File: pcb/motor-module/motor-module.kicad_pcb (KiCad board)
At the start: 2 copper layers, 37 x 27 mm, 9 parts, among them J1 Connector_male, J2 Screw_Terminal_01x02, K1 AZ822-2C-5DSE Signal-Relais, 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, Q1 2N 2222A SMD Bipolartransisto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

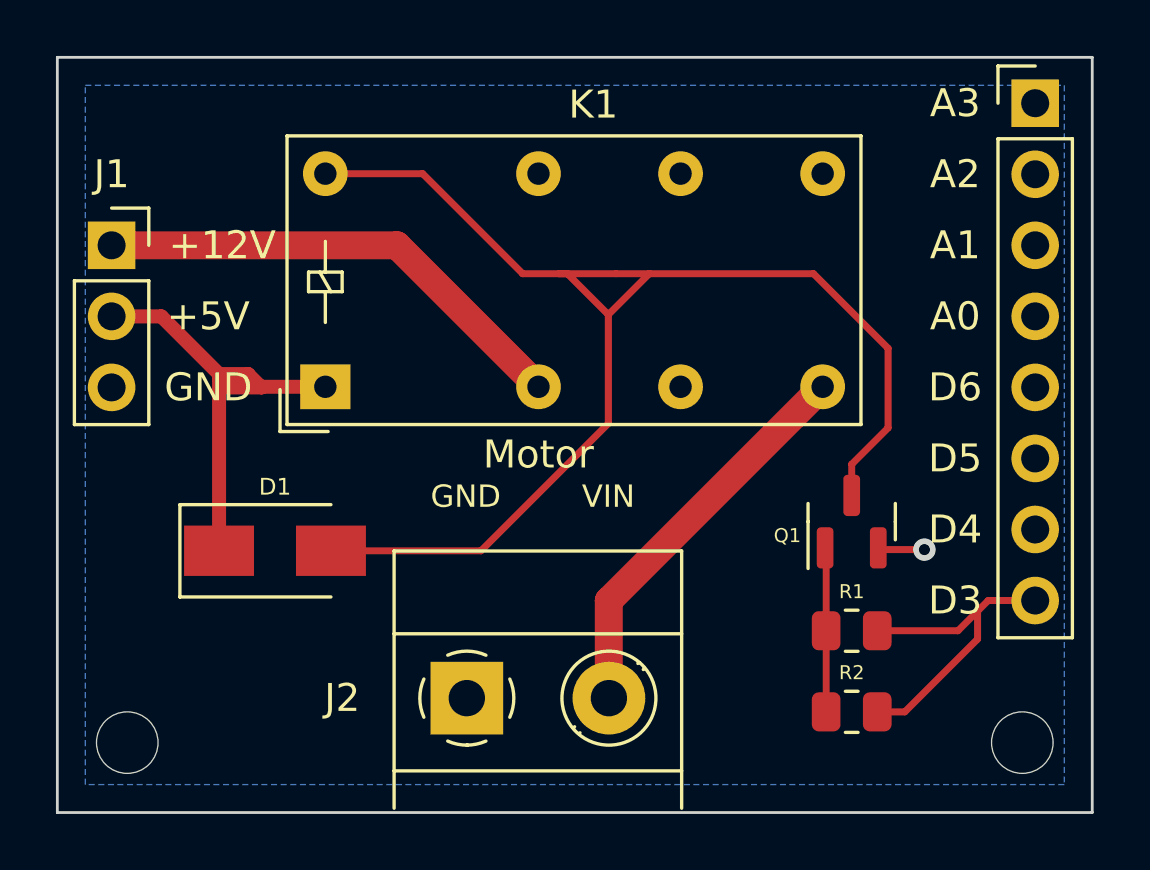
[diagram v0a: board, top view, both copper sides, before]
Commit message: pcb update
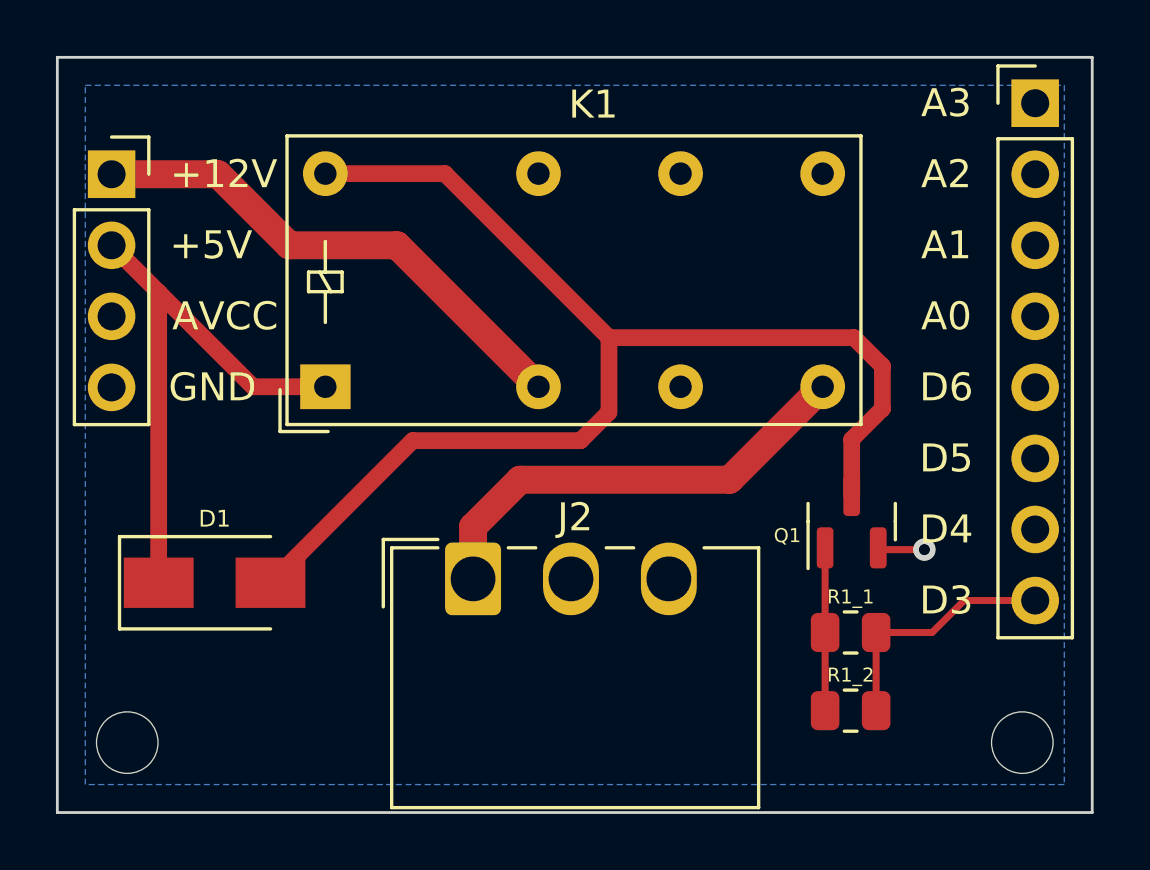
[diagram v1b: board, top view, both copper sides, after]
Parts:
- removed R1, R2: 1k, Resistor_SMD:R_0805_2012Metric
- added R1_1: 1k, Resistor_SMD:R_0805_2012Metric, F.Cu at (168.7, 110.4)
- added R1_2: 1k, Resistor_SMD:R_0805_2012Metric, F.Cu at (168.7, 113.2)
- J1: value Connector_male -> Connector_male_4x8; footprint CAN_ATmega:Connector_male -> CAN_ATmega:Connector_male_4x8
- J2: value Screw_Terminal_01x02 -> Screw_Terminal_01x03; footprint TerminalBlock_Phoenix:TerminalBlock_Phoenix_MKDS-1,5-2-5.08_1x02_P5.08mm_Horizontal -> Connector_Wago:Wago_734-163_1x03_P3.50mm_Horizontal
- moved J2 4.27 mm to (155.2, 108.4)
- moved D1 2.44 mm to (145.9, 108.6)
- moved J1 1.27 mm to (158.8, 99.1)
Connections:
- J1 pad 3: GND -> unconnected-(J1-Pad3)
- J1 pad 4: CMD -> GND
- J1 pad 5: unconnected-(J1-Pad5) -> CMD
- J2 pad 1: GND -> mot
- J2 pad 2: mot -> unconnected-(J2-Pad2)
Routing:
- net /sw-: track 48.6 -> 45.1 mm
- net +5V: track 16.7 -> 20.1 mm
- net CMD: track 11.8 -> 8.95 mm
- net mot: track 14.3 -> 16.4 mm
- net +12V: track 17.4 -> 18.4 mm
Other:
- board text removed: "GND"
- board text removed: "Motor"
- board text removed: "VIN"
